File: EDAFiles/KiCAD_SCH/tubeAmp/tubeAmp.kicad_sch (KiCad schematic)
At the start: 48 parts, among them J1 691137710002, J2 702471054, J3 691137710002, Q1 VPP12-800, U1 ECC88, U2 ECC88, U3 7591s

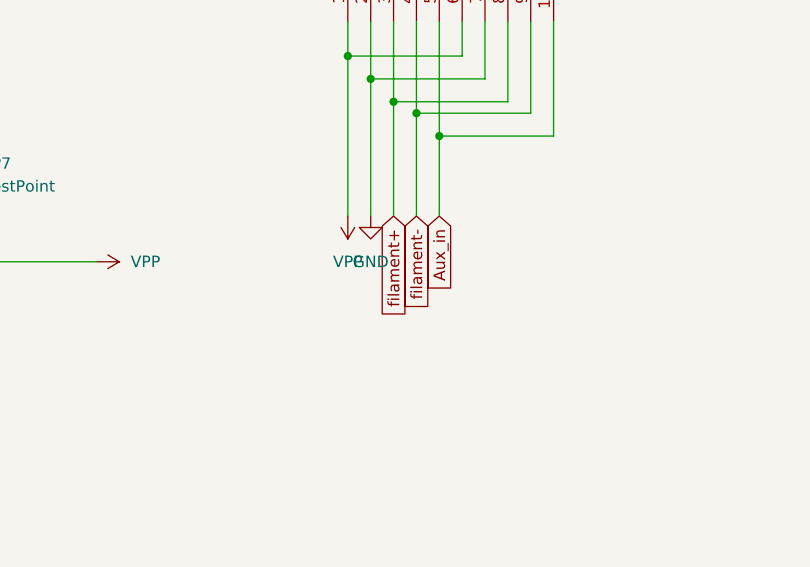
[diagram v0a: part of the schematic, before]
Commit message: Periodic Update from local Machine
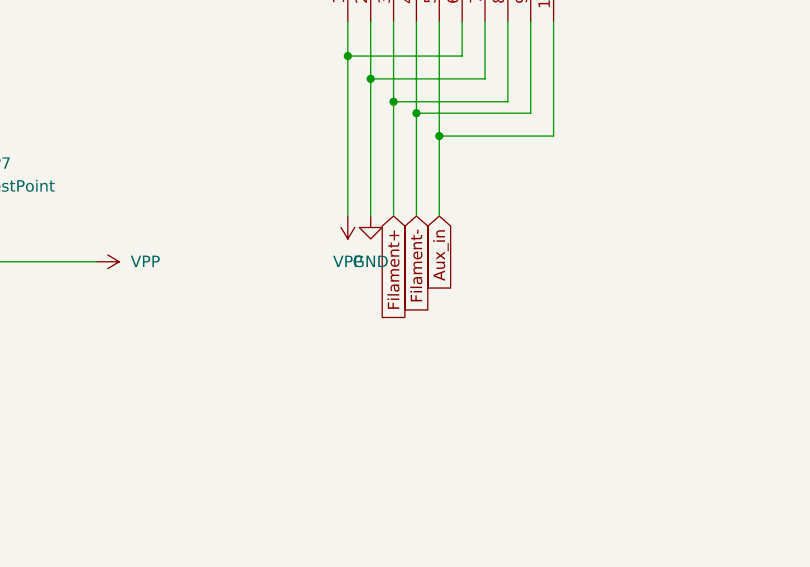
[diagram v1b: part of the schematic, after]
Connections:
- net filament+ is gone; now on net Filament+: J2.3, J2.8
- net filament- is gone; now on net Filament-: J2.4, J2.9
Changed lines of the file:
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@@
 		)
 	)
-	(global_label "filament-"
+	(global_label "Filament-"
 		(shape input)
 		(at 224.79 194.31 270)
@@
 		)
 		(property "Intersheetrefs" "${INTERSHEET_REFS}"
-			(at 224.79 206.6689 90)
+			(at 224.79 207.0318 90)
 			(effects
 				(font
@@
 		)
 	)
-	(global_label "filament+"
+	(global_label "Filament+"
 		(shape input)
 		(at 222.25 194.31 270)
@@
 		)
 		(property "Intersheetrefs" "${INTERSHEET_REFS}"
-			(at 222.25 206.6689 90)
+			(at 222.25 207.0318 90)
 			(effects
 				(font
